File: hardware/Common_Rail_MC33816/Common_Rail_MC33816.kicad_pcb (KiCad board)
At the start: 4 copper layers, 101.6 x 119.6 mm, 183 parts, among them J10 INJ_Term, J11 INJ_Term, J12 INJ_Term, J14 CONN_01X03, J15 CONN_01X01, J20 Conn_01x02, J3 CONN_02X08, J4 CONN_02X08, J5 CONN_01X03, J6 CONN_01X03, J7 CONN_01X03, J8 INJ_Term, J9 INJ_Term, Q1 BUK9230-100B, Q10 BUK9230-100B, Q11 BUK9230-100B, Q12 BUK9230-100B, Q2 BUK9230-100B, Q3 BUK9230-100B, Q4 BUK9230-100B, Q5 BUK9230-100B, Q6 BUK9230-100B, Q7 BUK9230-100B, Q8 BUK9230-100B, Q9 BUK9230-100B, U4 MC33816, Y1 1MHz, Y2 1MHz

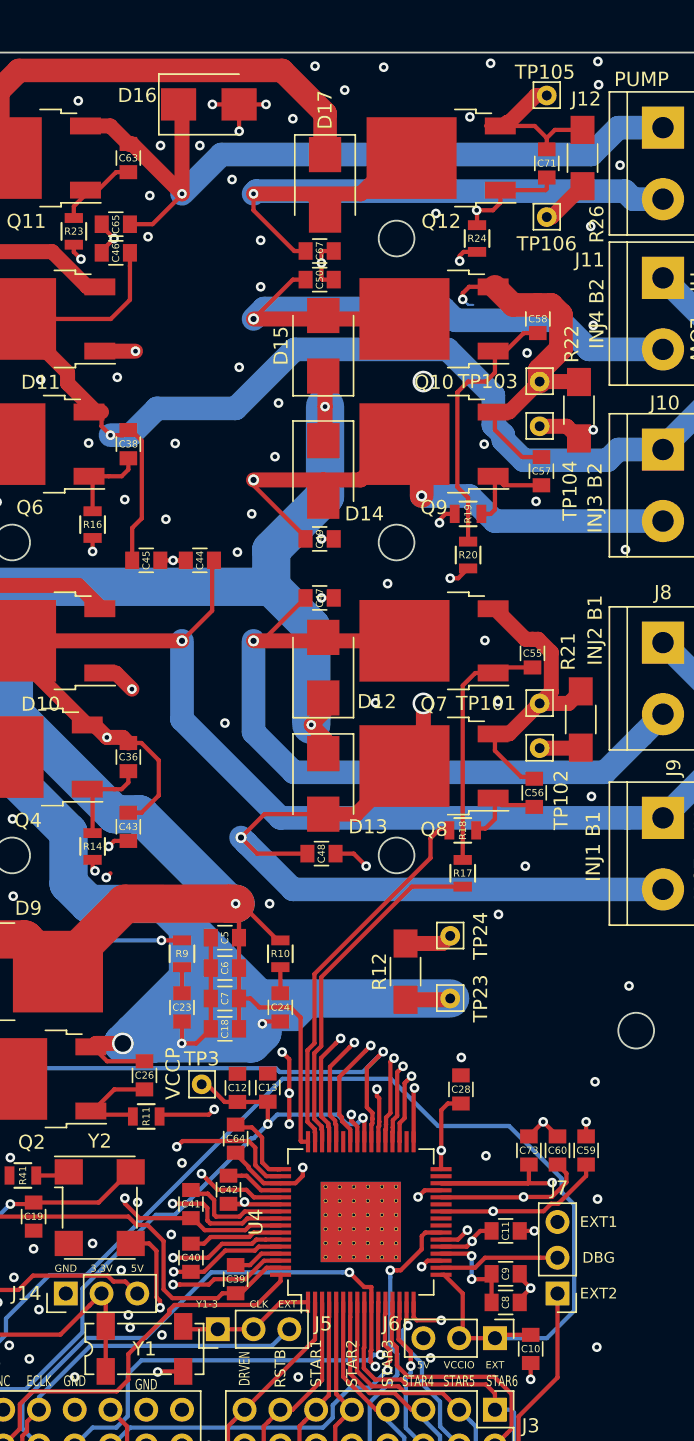
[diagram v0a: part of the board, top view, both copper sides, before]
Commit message: update pcb files
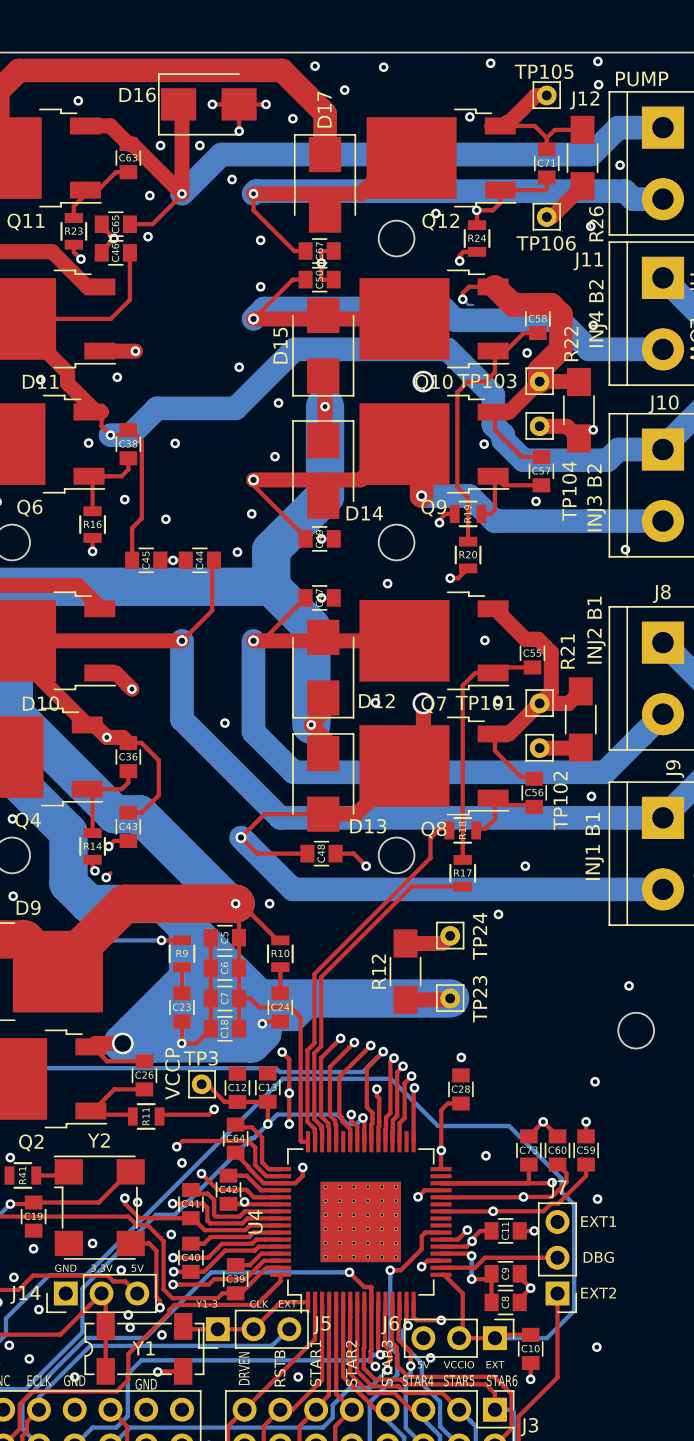
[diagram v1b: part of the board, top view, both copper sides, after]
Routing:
- added copper zone on In1.Cu, net GND
- added copper zone on In2.Cu, net GND
- removed copper zone on GND, net GND
- removed copper zone on PWR_AN, net GND
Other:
- net class 1A_external removed
- net class 2.5A_external removed
- net class 3.5A_external removed
- net class 3.5A_external_high_voltage removed
- net class 5A_external removed
- net class Default removed
- net class Supply_200V removed
- net class min2_extern_.188A removed
- net class min_extern_.241A removed
